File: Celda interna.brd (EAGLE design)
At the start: 92.5 x 55.4 mm, 19 parts, among them U1 ATMEGA328P_PDIP, X2 2510-

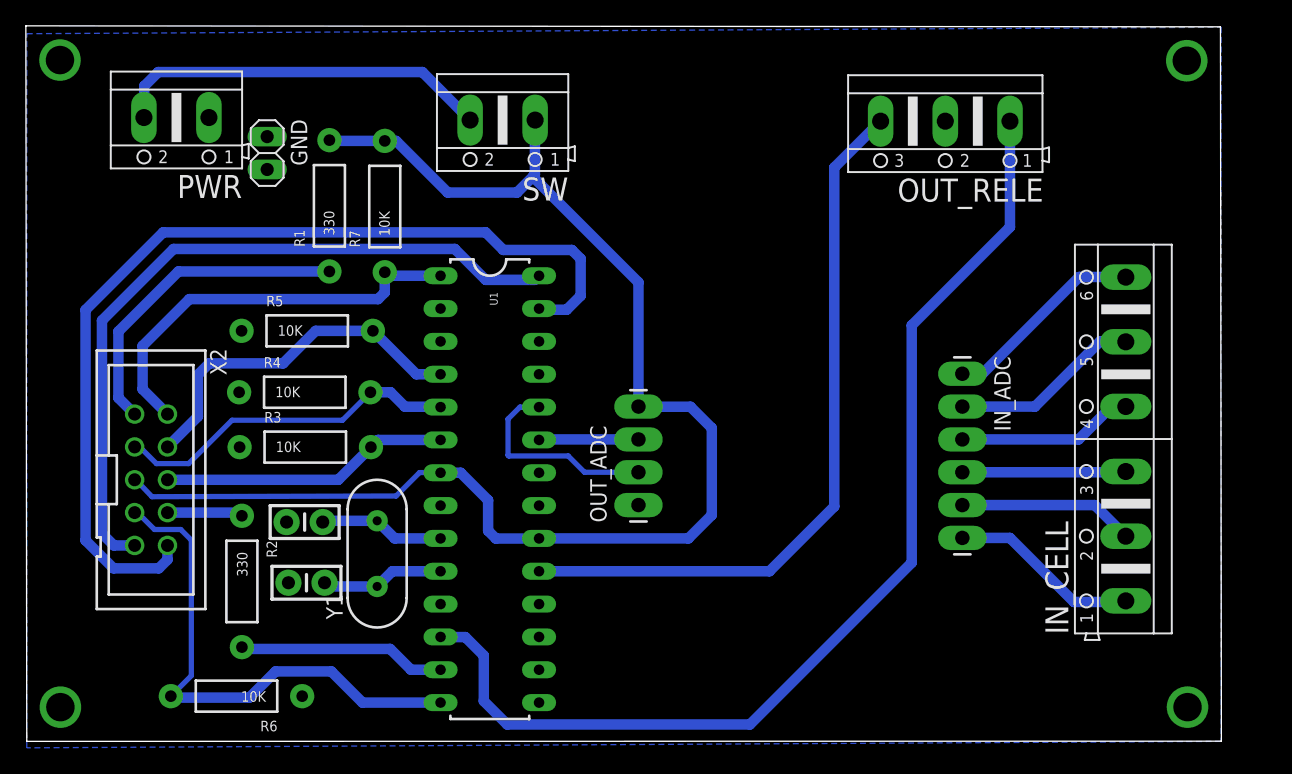
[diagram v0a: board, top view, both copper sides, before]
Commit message: Update logo
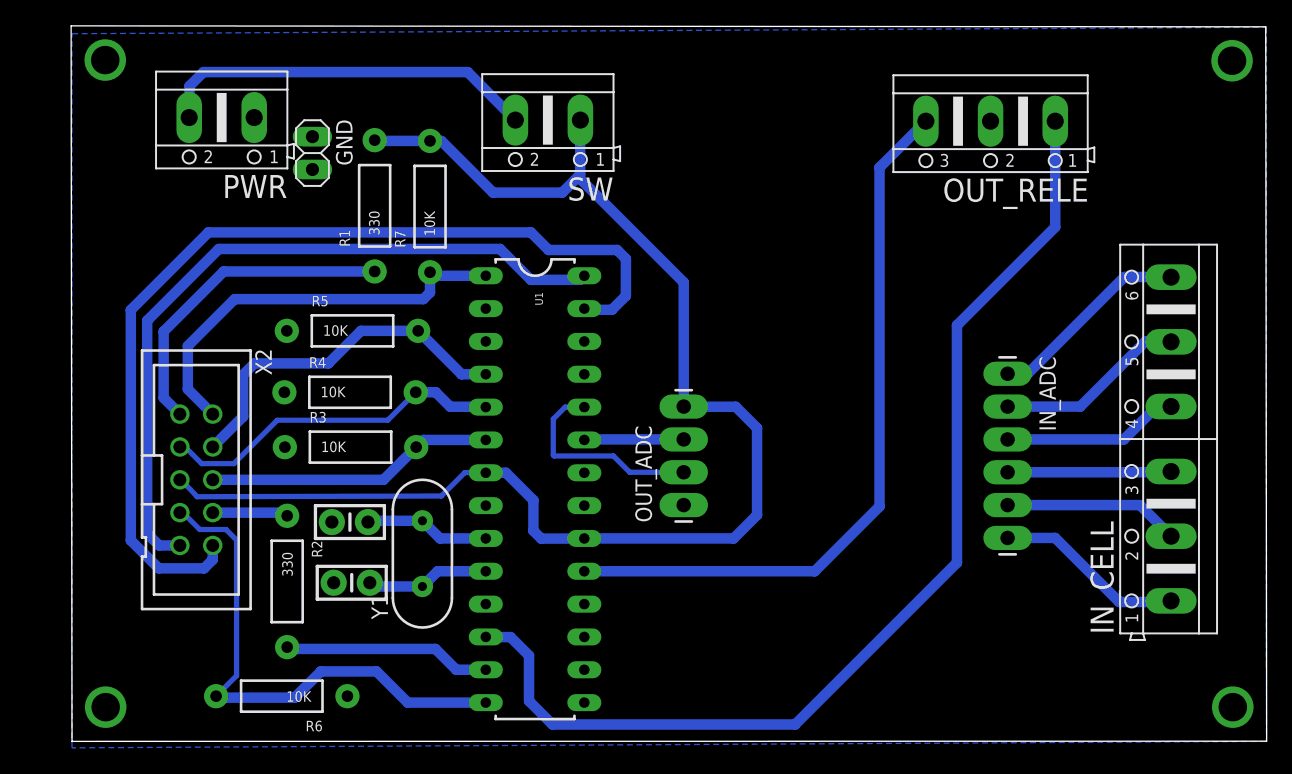
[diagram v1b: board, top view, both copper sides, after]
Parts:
- moved C2 3.50 mm to (21.6, 12.3)
- moved IN_ADC 3.50 mm to (72.4, 28.4)
- moved IN_CELL 3.50 mm to (85.0, 23.4)
- moved OUT_ADC 3.50 mm to (47.3, 18.3)
- moved OUT_RELE 3.50 mm to (71.1, 48.0)
- moved R1 3.50 mm to (23.4, 41.4)
- moved R2 3.50 mm to (16.6, 12.4)
- moved R3 3.50 mm to (21.5, 22.8)
- moved R5 3.50 mm to (21.7, 31.8)
- moved R6 3.50 mm to (16.2, 3.50)
- moved R7 3.50 mm to (27.7, 41.4)
- moved SW 3.50 mm to (36.8, 48.1)
- moved U1 3.50 mm to (35.8, 19.5)
- moved Y1 3.50 mm to (27.1, 14.5)
- moved X2 3.50 mm to (9.62, 20.2)
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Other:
- board text added: "C:/Users/Jose/Pictures/JoseM.bmp"
